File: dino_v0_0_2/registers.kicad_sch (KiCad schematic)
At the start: 14 parts, among them U31 74LS373, U32 74LS373, U33 74LS373, U35 74LS373, U41 74LS245, U42 74LS245, U43 74LS245, U44 74LS245, U45 74LS121, U46 74LS121, U47 74LS04, U48 74LS00, U49 74LS04, U50 74LS02

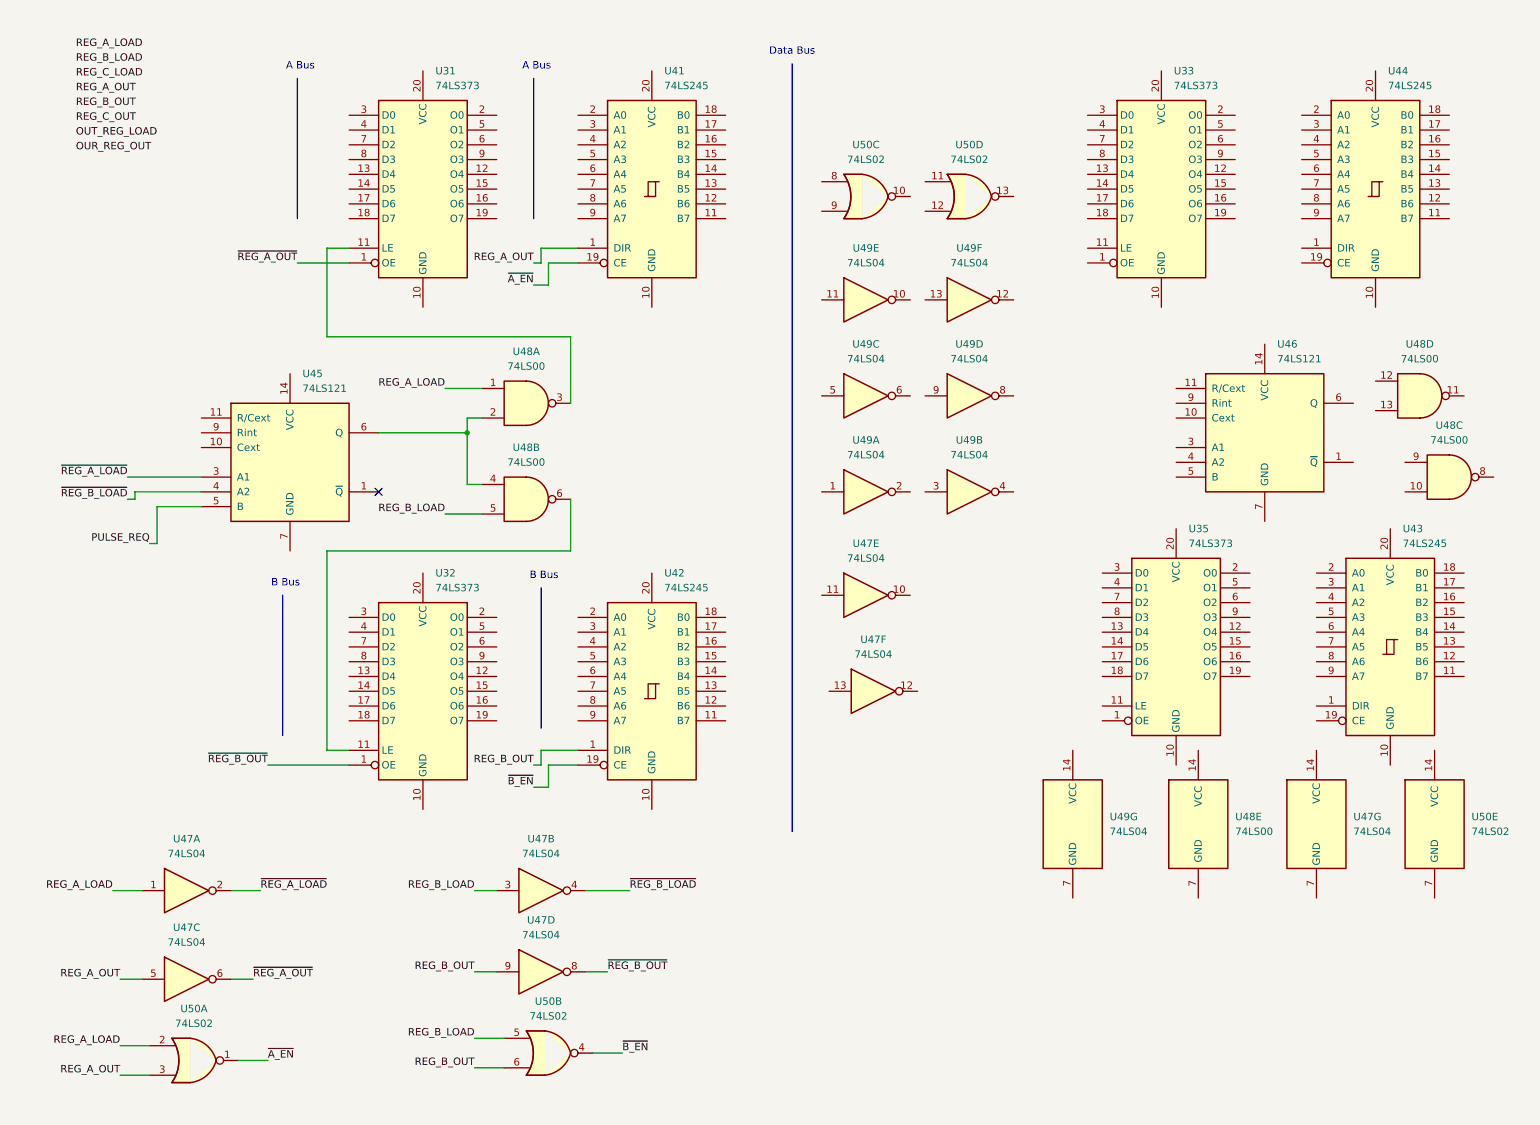
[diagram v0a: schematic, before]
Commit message: KiCAD Updates
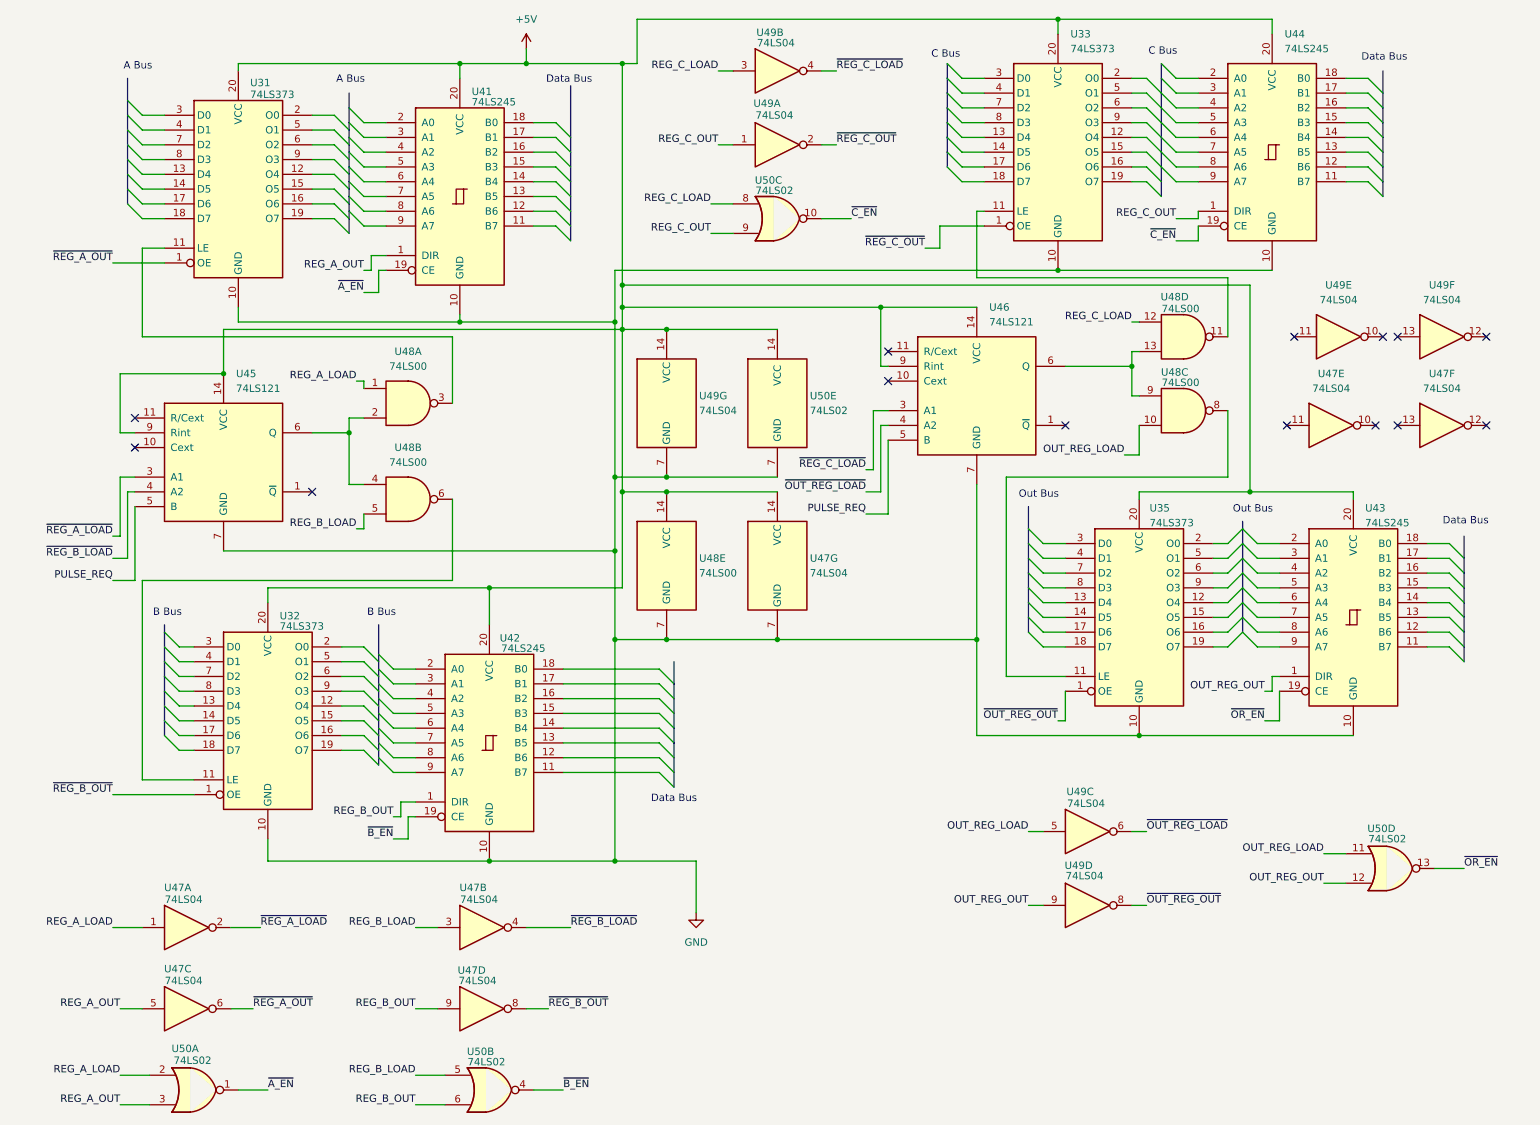
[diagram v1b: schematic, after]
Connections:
- net OUT_REG_LOAD: now also U48.10, U49.5, U50.11
- net PULSE_REQ: now also U46.5 (B)
- net REG_C_LOAD: now also U48.12, U49.3, U50.8
- net REG_C_OUT: now also U44.1 (DIR), U49.1, U50.9
- net GND: now reaches U41.10 (GND)
- net GND: now also U31.10 (GND), U32.10 (GND), U33.10 (GND), U35.10 (GND), U42.10 (GND), U43.10 (GND), U44.10 (GND), U45.7 (GND), U46.7 (GND), U47.7 (GND), U48.7 (GND), U49.7 (GND), U50.7 (GND)
- net +5V: now reaches U41.20 (VCC)
- net +5V: now also U31.20 (VCC), U32.20 (VCC), U33.20 (VCC), U35.20 (VCC), U42.20 (VCC), U43.20 (VCC), U44.20 (VCC), U45.14 (VCC), U45.9 (Rint), U46.14 (VCC), U46.9 (Rint), U47.14 (VCC), U48.14 (VCC), U49.14 (VCC), U50.14 (VCC)
- net ~{OUT_REG_LOAD}: now reaches U49.6
- net ~{OUT_REG_LOAD}: now also U46.4 (A2)
- net ~{REG_C_LOAD}: now reaches U49.4
- net ~{REG_C_LOAD}: now also U46.3 (A1)
- net ~{OUT_REG_OUT}: now reaches U49.8
- net ~{OUT_REG_OUT}: now also U35.1 (OE)
- net OUT_REG_OUT: now reaches U49.9
- net OUT_REG_OUT: now also U43.1 (DIR), U50.12
- net ~{REG_C_OUT}: now reaches U33.1 (OE)
- net ~{REG_C_OUT}: now also U49.2
- net at U33.11 (LE): now also U48.11
- net ~{C_EN}: now reaches U44.19 (CE)
- net ~{C_EN}: now also U50.10
- net at U48.13: now also U46.6 (Q), U48.9
- net ~{OR_EN}: now reaches U50.13
- net ~{OR_EN}: now also U43.19 (CE)
- net at U35.11 (LE): now also U48.8
- no-connect marks 1 -> 14
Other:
- note added: "C Bus"
- note added: "Out Bus"
- moved on the sheet: U31, U32, U33, U35, U41, U42, U43, U44, U45, U46, U47A, U47B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
